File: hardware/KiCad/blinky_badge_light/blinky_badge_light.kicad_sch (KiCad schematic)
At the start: 9 parts, among them U1 ESP32-S3-WROOM-1

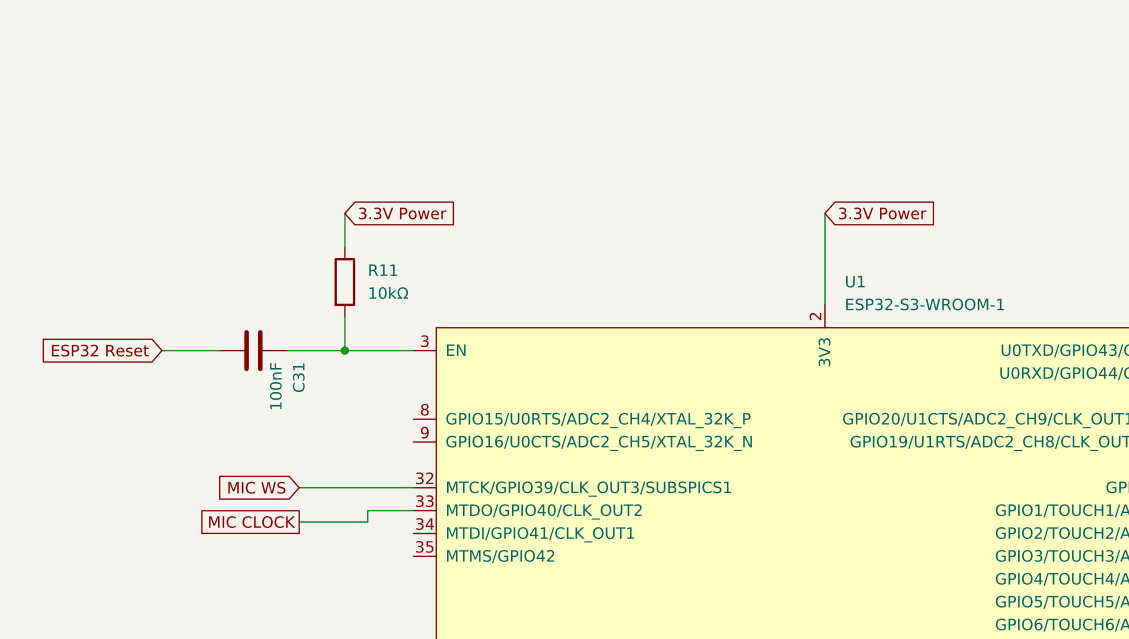
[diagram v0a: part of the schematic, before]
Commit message: updates to hardware schematic
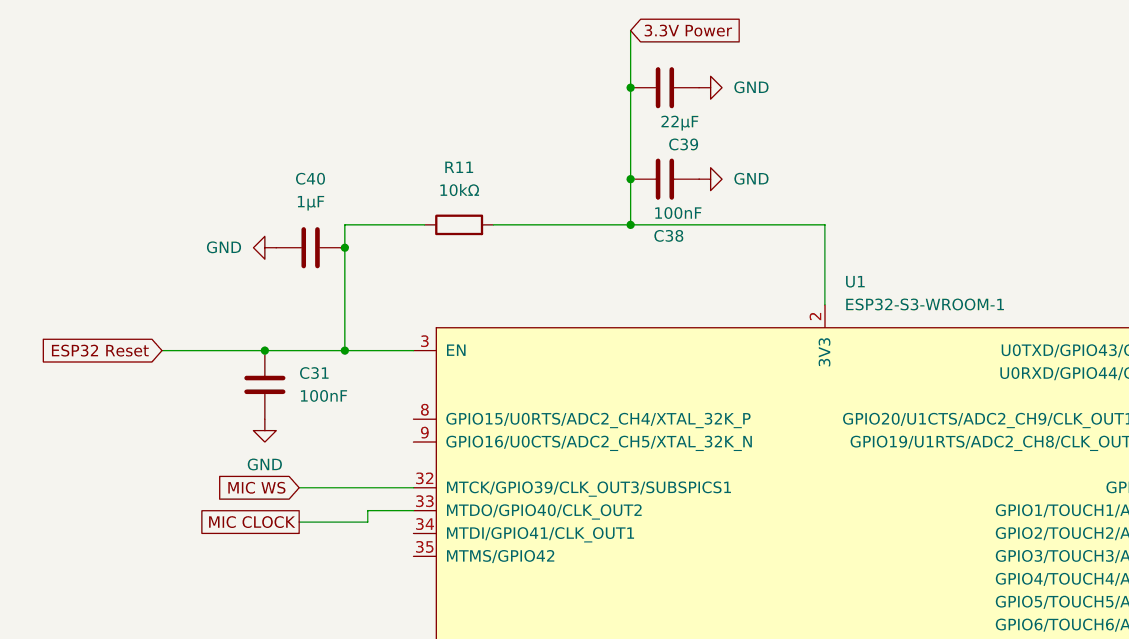
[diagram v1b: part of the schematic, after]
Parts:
- added C38: 100nF, Capacitor_SMD:C_0402_1005Metric, symbol Device:C
- added C39: 22µF, Capacitor_SMD:C_0201_0603Metric, symbol Device:C
- added C40: 1µF, Capacitor_SMD:C_0603_1608Metric, symbol Device:C
- C31: footprint Capacitor_SMD:C_0402_1005Metric -> Resistor_SMD:R_0402_1005Metric
- U1: footprint PCM_Espressif:ESP32-S3-WROOM-1 -> RF_Module:ESP32-S3-WROOM-1
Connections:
- net 3.3V Power: now also R11.2, C38.2, C39.1; no longer R11.1
- net ESP32 Reset: now also R11.1, U1.3 (EN), C40.2
- net GND: now also C31.1, C38.1, C39.2, C40.1
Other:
- moved on the sheet: R11

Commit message: hardware updates, gitignore to ignore backups
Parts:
- TOUCH_1, TOUCH_2, TOUCH_3, TOUCH_4: footprint TestPoint:TestPoint_Pad_D4.0mm -> footprints:TestPoint_Pad_D12.0mm
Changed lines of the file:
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@@
 			)
 		)
-		(property "Footprint" "TestPoint:TestPoint_Pad_D4.0mm"
+		(property "Footprint" "footprints:TestPoint_Pad_D12.0mm"
 			(at 234.95 100.33 0)
 			(effects
@@
 			)
 		)
-		(property "Footprint" "TestPoint:TestPoint_Pad_D4.0mm"
+		(property "Footprint" "footprints:TestPoint_Pad_D12.0mm"
 			(at 234.95 107.95 0)
 			(effects
@@
 			)
 		)
-		(property "Footprint" "TestPoint:TestPoint_Pad_D4.0mm"
+		(property "Footprint" "footprints:TestPoint_Pad_D12.0mm"
 			(at 234.95 92.71 0)
 			(effects
@@
 			)
 		)
-		(property "Footprint" "TestPoint:TestPoint_Pad_D4.0mm"
+		(property "Footprint" "footprints:TestPoint_Pad_D12.0mm"
 			(at 234.95 85.09 0)
 			(effects

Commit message: stuff from today
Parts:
- C39: footprint Capacitor_SMD:C_0201_0603Metric -> Capacitor_SMD:C_0603_1608Metric
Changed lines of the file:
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@@
 			)
 		)
-		(property "Footprint" "Capacitor_SMD:C_0201_0603Metric"
+		(property "Footprint" "Capacitor_SMD:C_0603_1608Metric"
 			(at 132.08 29.5148 0)
 			(effects

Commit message: fix some stuff with the footprints, rearrange some things
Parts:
- C31: footprint Resistor_SMD:R_0402_1005Metric -> Capacitor_SMD:C_0402_1005Metric
- TOUCH_4: footprint footprints:TestPoint_Pad_D12.0mm -> TestPoint:TestPoint_Pad_D4.0mm
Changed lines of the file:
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@@
 			)
 		)
-		(property "Footprint" "footprints:TestPoint_Pad_D12.0mm"
+		(property "Footprint" "TestPoint:TestPoint_Pad_D4.0mm"
 			(at 234.95 107.95 0)
 			(effects
@@
 			)
 		)
-		(property "Footprint" "Resistor_SMD:R_0402_1005Metric"
+		(property "Footprint" "Capacitor_SMD:C_0402_1005Metric"
 			(at 82.8548 59.69 0)
 			(effects

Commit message: pad 4 is now stop sign shaped since its the off button
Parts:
- TOUCH_4: footprint TestPoint:TestPoint_Pad_D4.0mm -> footprints:Touch_Pad_StopSign_6mm
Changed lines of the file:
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@@
 			)
 		)
-		(property "Footprint" "TestPoint:TestPoint_Pad_D4.0mm"
+		(property "Footprint" "footprints:Touch_Pad_StopSign_6mm"
 			(at 234.95 107.95 0)
 			(effects
